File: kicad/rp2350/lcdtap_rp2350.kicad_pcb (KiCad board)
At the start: 2 copper layers, 122 x 50 mm, 116 parts, among them J1 HDMI-001S, J2 Conn_02x08_Odd_Even, J3 Conn_01x03, J4 Conn_02x08_Odd_Even, J5 Conn_02x04_Odd_Even, P1 TYPE-C16PIN, SW1 SKRPACE010, SW2 SKRPACE010, SW3 SSSS811101, SW4 SKRPACE010, SW5 SKRPACE010, SW6 SKRPACE010, SW7 SKRPACE010, SW8 SKRPACE010, U1 RP2350A, U2 W25Q32JVSSIQ, U3 AP63203WU, U4 74HC595, U5 74HC4040, U6 74LVC1G04, Y1 ABM8-272-T3

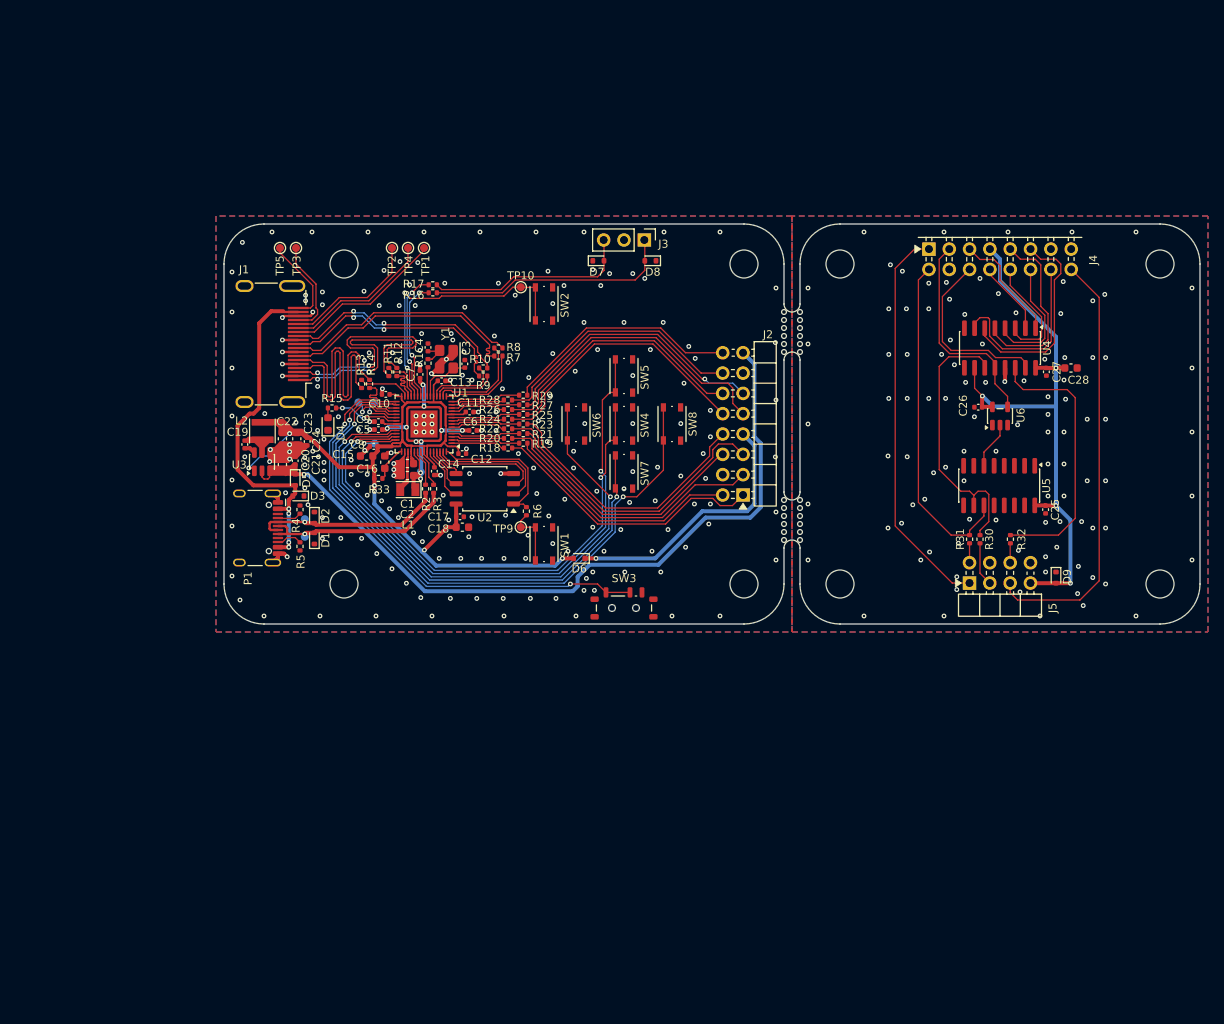
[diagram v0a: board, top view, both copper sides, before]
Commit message: PCB artwork draft
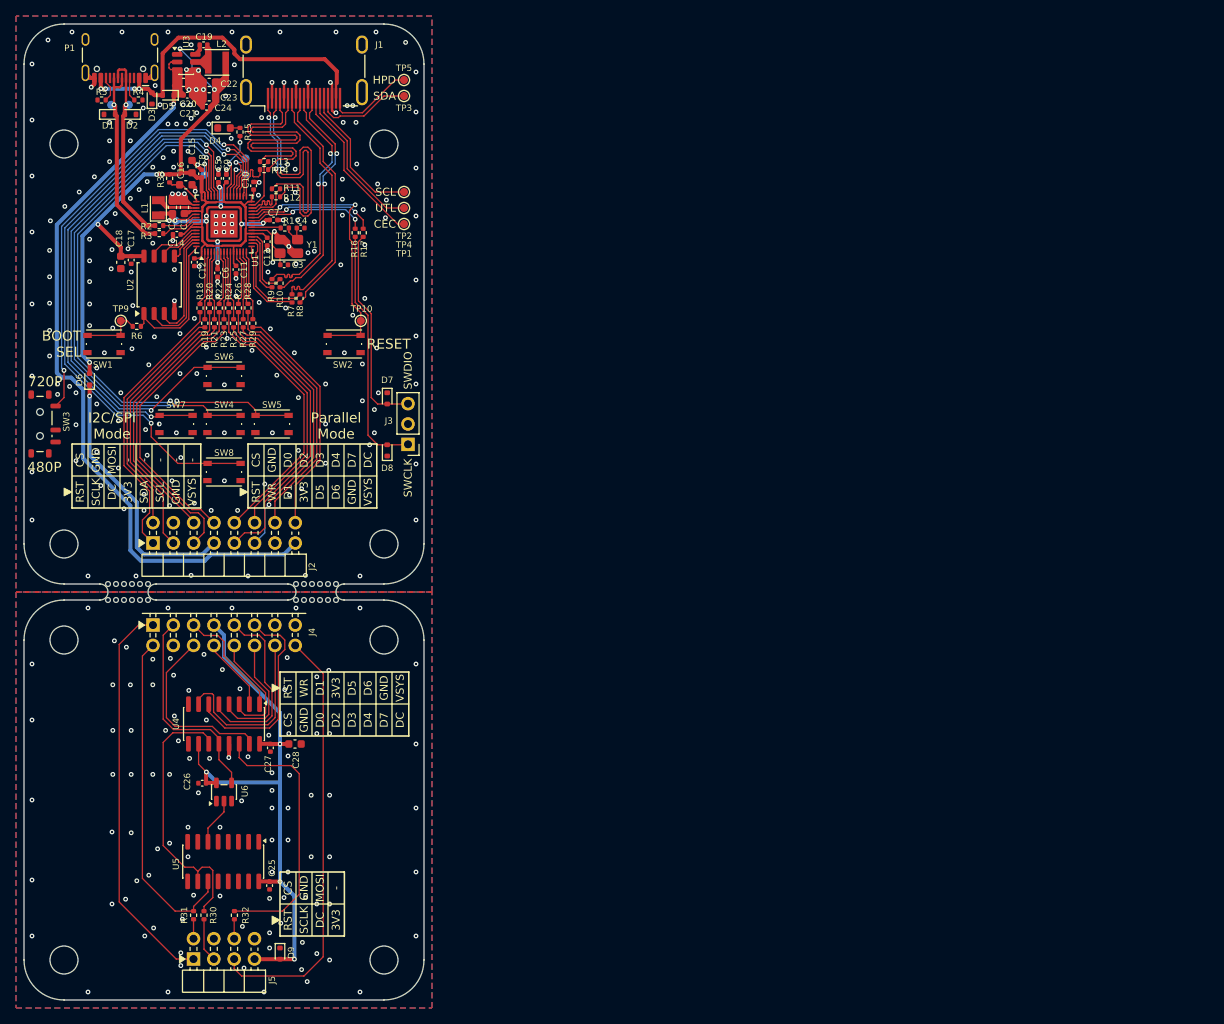
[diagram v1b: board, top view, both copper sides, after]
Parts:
- moved C27 107.8 mm to (65.8, 125.5)
- moved R32 107.8 mm to (61.3, 146.4)
- moved C26 107.8 mm to (57.3, 129.9)
- moved C28 107.8 mm to (68.9, 125.0)
- moved D9 107.8 mm to (67.0, 151.2)
- moved H5 107.8 mm to (40.0, 112.0)
- moved H6 107.8 mm to (40.0, 152.0)
- moved H7 107.8 mm to (80.0, 112.0)
- moved H8 107.8 mm to (80.0, 152.0)
- moved J4 107.8 mm to (68.9, 112.7)
- moved J5 107.8 mm to (63.8, 149.3)
- moved R30 107.8 mm to (57.5, 146.4)
- moved U4 107.8 mm to (60.0, 122.5)
- moved U5 107.8 mm to (59.9, 139.7)
- moved U6 107.8 mm to (60.0, 131.0)
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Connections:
- SW3 pad 2: /SW_720P -> GND
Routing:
- net /SW_720P: track 60.8 -> 57.8 mm
- net Net-(J1-HPD): track 10.8 -> 11.3 mm
- net Net-(J1-UTILITY): track 18.9 -> 19.4 mm
- net Net-(J1-SDA): track 12.1 -> 12.6 mm
- net Net-(J1-SCL): track 17.5 -> 18.0 mm
- net Net-(J1-CEC): track 20.2 -> 20.7 mm
- net GND: vias 218 -> 219
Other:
- board size 122 x 50 mm -> 50 x 122 mm
- board text added: "-"
- board text added: "1V1"
- board text added: "3V3"
- board text added: "480P"
- board text added: "720P"
- board text added: "BOOT SEL"
- board text added: "CEC"
- board text added: "CS"
- board text added: "D+"
- board text added: "D-"
- board text added: "D0"
- board text added: "D1"
- board text added: "D2"
- board text added: "D3"
- board text added: "D4"
- board text added: "D5"
- board text added: "D6"
- board text added: "D7"
- board text added: "DC"
- board text added: "GND"
- board text added: "GPIO23"
- board text added: "GPIO24"
- board text added: "GPIO29"
- board text added: "HPD"
- board text added: "I2C/SPI Mode"
- board text added: "MOSI"
- board text added: "Parallel Mode"
- board text added: "RESET"
- board text added: "RST"
- board text added: "SCL"
- board text added: "SCLK"
- board text added: "SDA"
- board text added: "SWCLK"
- board text added: "SWDIO"
- board text added: "UTL"
- board text added: "VSYS"
- board text added: "WR"
